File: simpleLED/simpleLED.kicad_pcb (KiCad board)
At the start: 2 copper layers, 28 x 18 mm, 4 parts, among them J1 USB_A, SW1 SW_Push

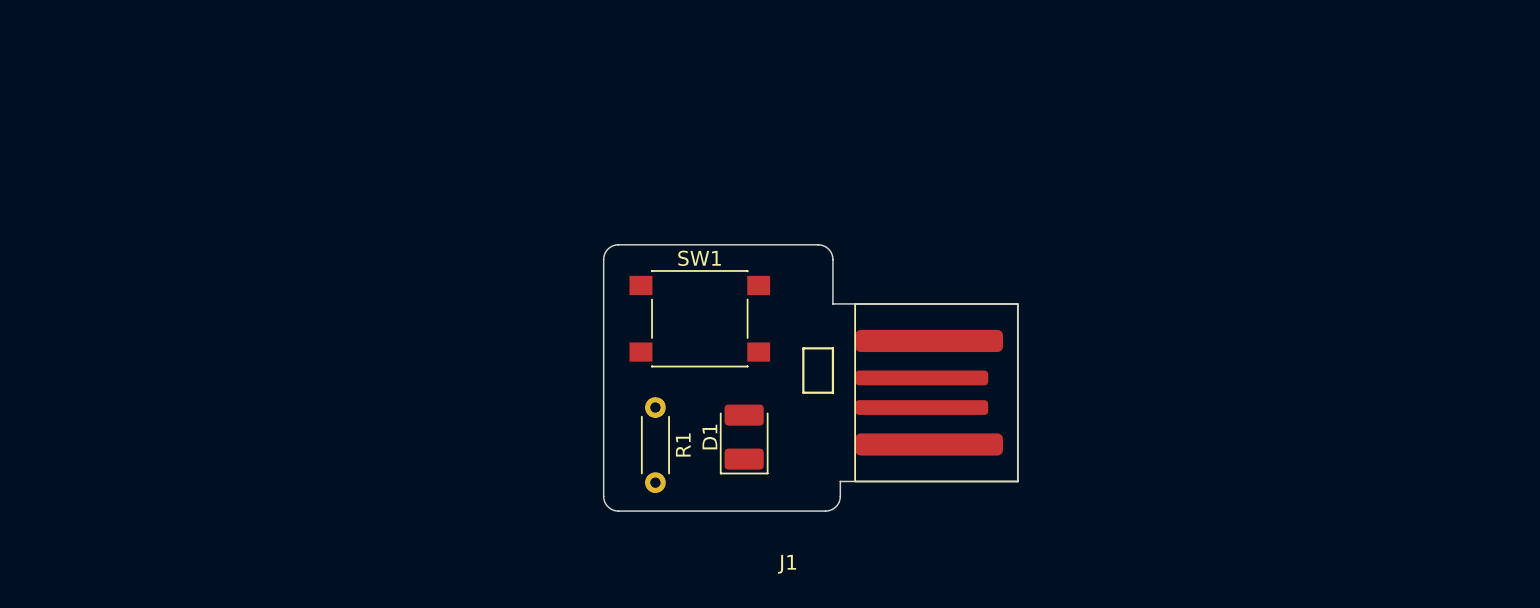
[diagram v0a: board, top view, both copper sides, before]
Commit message: updated
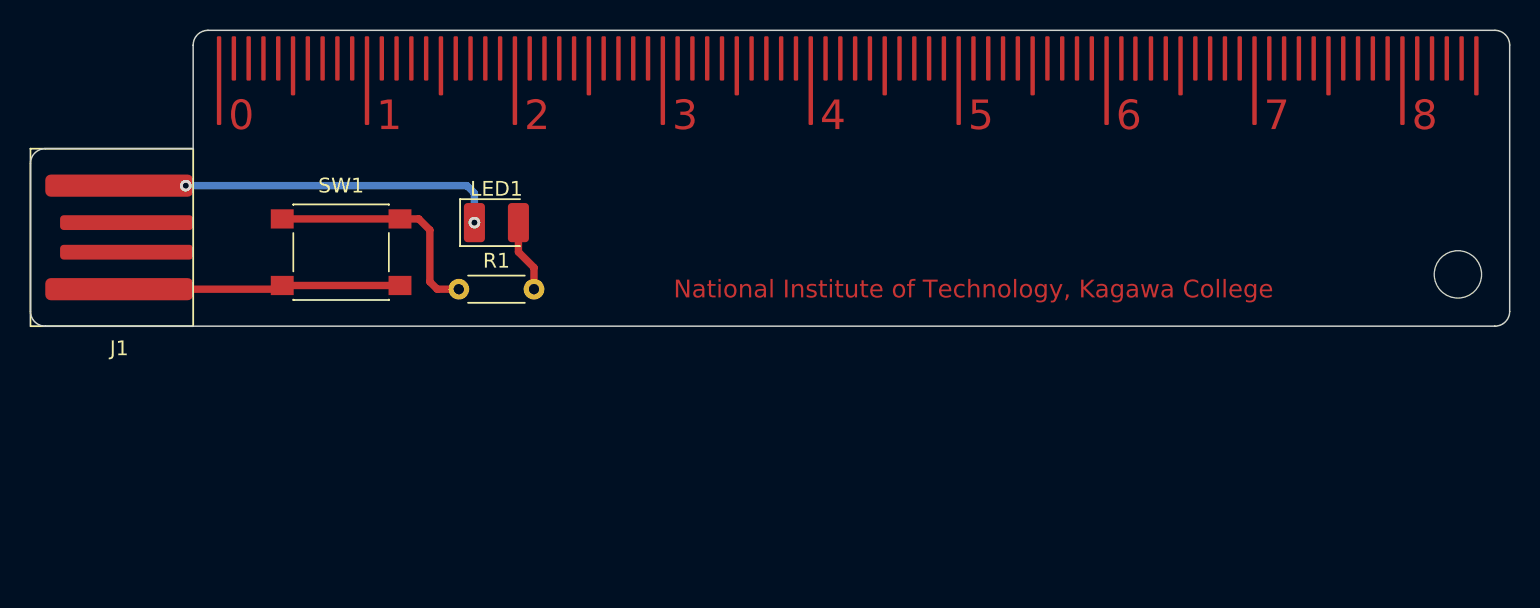
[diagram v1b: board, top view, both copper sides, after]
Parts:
- removed D1: LED, Diode_SMD:D_1210_3225Metric_Pad1.42x2.65mm_HandSolder
- added LED1: LED, Diode_SMD:D_1210_3225Metric_Pad1.42x2.65mm_HandSolder, F.Cu at (50.2, 32.5)
- added REF**: ruler, simpleLED:ruler, F.Cu at (71.5, 25.8)
- added REF**: MountingHole_3.2mm_M3, MountingHole:MountingHole_3.2mm_M3, F.Cu at (115.2, 36.0)
- moved J1 54.3 mm to (24.2, 33.5), turned to 0 degrees
- moved SW1 24.7 mm to (39.8, 34.5), turned to 180 degrees
- moved R1 15.5 mm to (47.7, 37.0), turned to 0 degrees
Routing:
- net GND: track 0.00 -> 26.2 mm, vias 0 -> 2
- net +5V: track 0.00 -> 19.1 mm
- net Net-(R1-Pad1): track 0.00 -> 16.0 mm
- net Net-(D1-Pad2): track 0.00 -> 4.94 mm
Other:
- board size 28 x 18 mm -> 100 x 20 mm
- board text added: "National Institute of Technology, Kagawa College"
